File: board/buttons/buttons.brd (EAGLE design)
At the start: 125 x 64.4 mm, 10 parts, among them J1 188275-8, Q1 MMBT4403, Q2 MMBT4403, Q3 MMBT4403

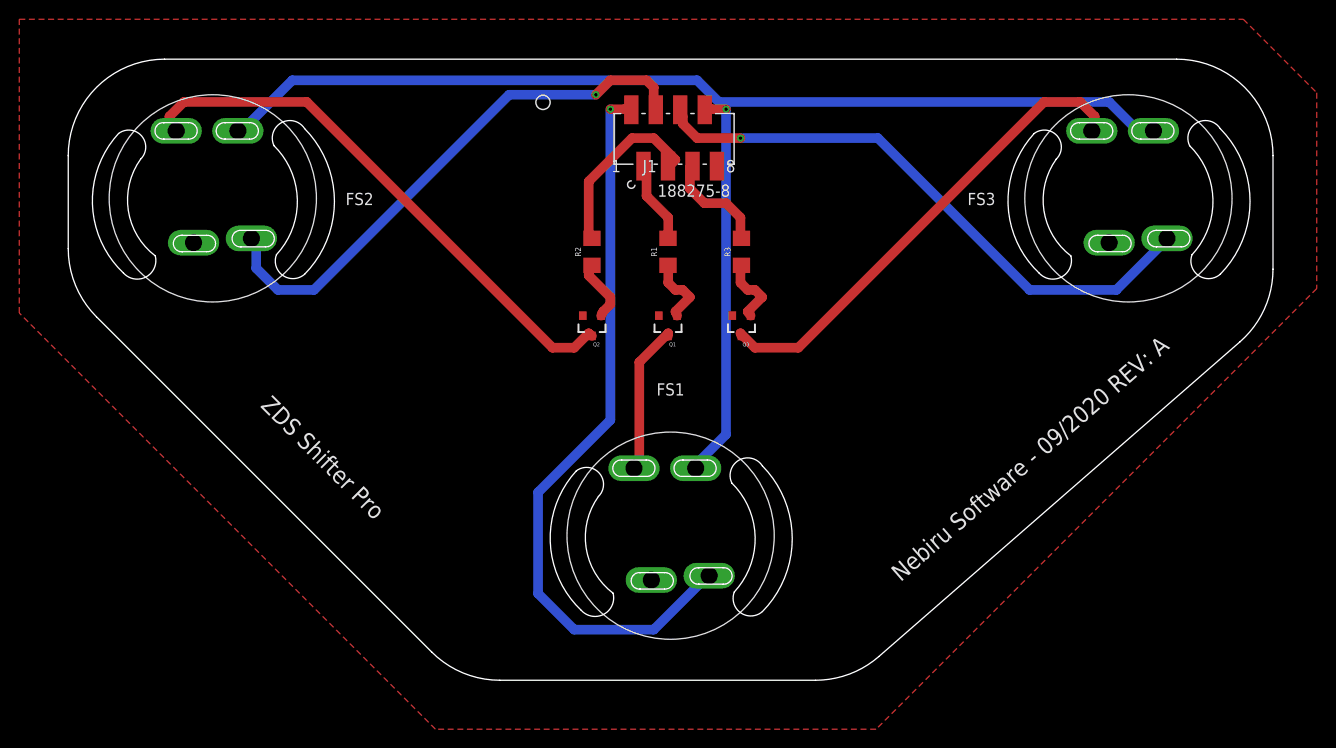
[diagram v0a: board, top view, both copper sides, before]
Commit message: board changes
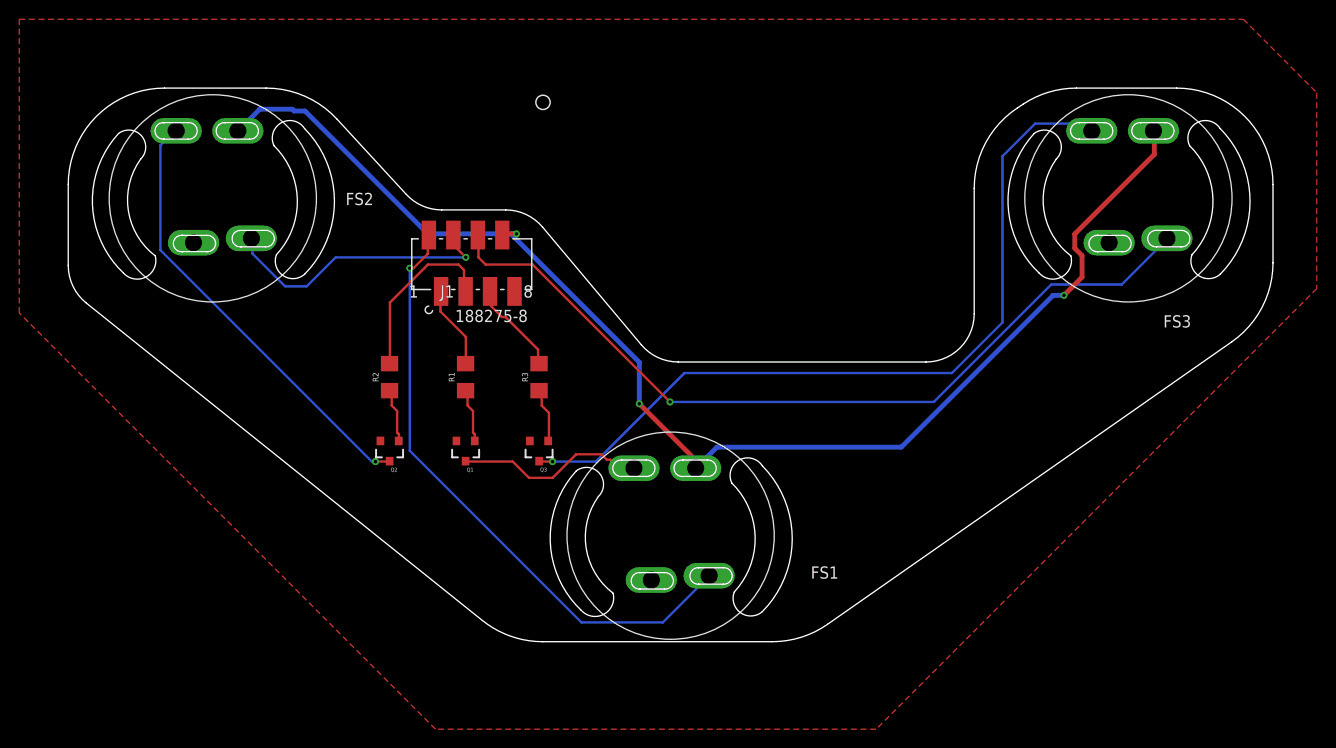
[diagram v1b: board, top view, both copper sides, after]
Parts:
- moved R1 24.7 mm to (41.2, 31.4)
- moved R2 24.7 mm to (33.3, 31.4)
- moved J1 24.7 mm to (37.4, 40.3)
- moved Q1 24.7 mm to (41.2, 23.8)
- moved Q2 24.7 mm to (33.3, 23.8)
- moved Q3 24.7 mm to (48.9, 23.8)
- moved R3 24.7 mm to (48.9, 31.4)
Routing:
- net FS3_LED-: track 50.6 -> 82.3 mm, vias 0 -> 1
- net FS2_BTN: track 57.5 -> 29.3 mm
- net FS3_BTN: track 61.1 -> 87.1 mm
- net FS1_BTN: track 77.1 -> 63.9 mm
- net FS2_LED-: track 57.9 -> 46.0 mm, vias 0 -> 1
- net VIN: track 141.1 -> 136.1 mm, vias 1 -> 3
- net FS1_LED-: track 15.8 -> 19.9 mm
- net N$10: track 7.33 -> 5.68 mm
- net N$2: track 7.25 -> 5.61 mm
- net FS3_LED: track 11.2 -> 9.84 mm
- net N$13: track 6.67 -> 5.62 mm
- net FS2_LED: track 18.9 -> 18.2 mm
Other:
- board size 125 x 64.4 mm -> 125 x 57.4 mm
- board text added: "Nebiru Software - 09/2020 REV: C"
- board text removed: "Nebiru Software - 09/2020 REV: A"
